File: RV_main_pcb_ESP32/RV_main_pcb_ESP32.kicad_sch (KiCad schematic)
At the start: 3 parts, among them J1 Conn_01x15_Female, J2 Conn_01x15_Female

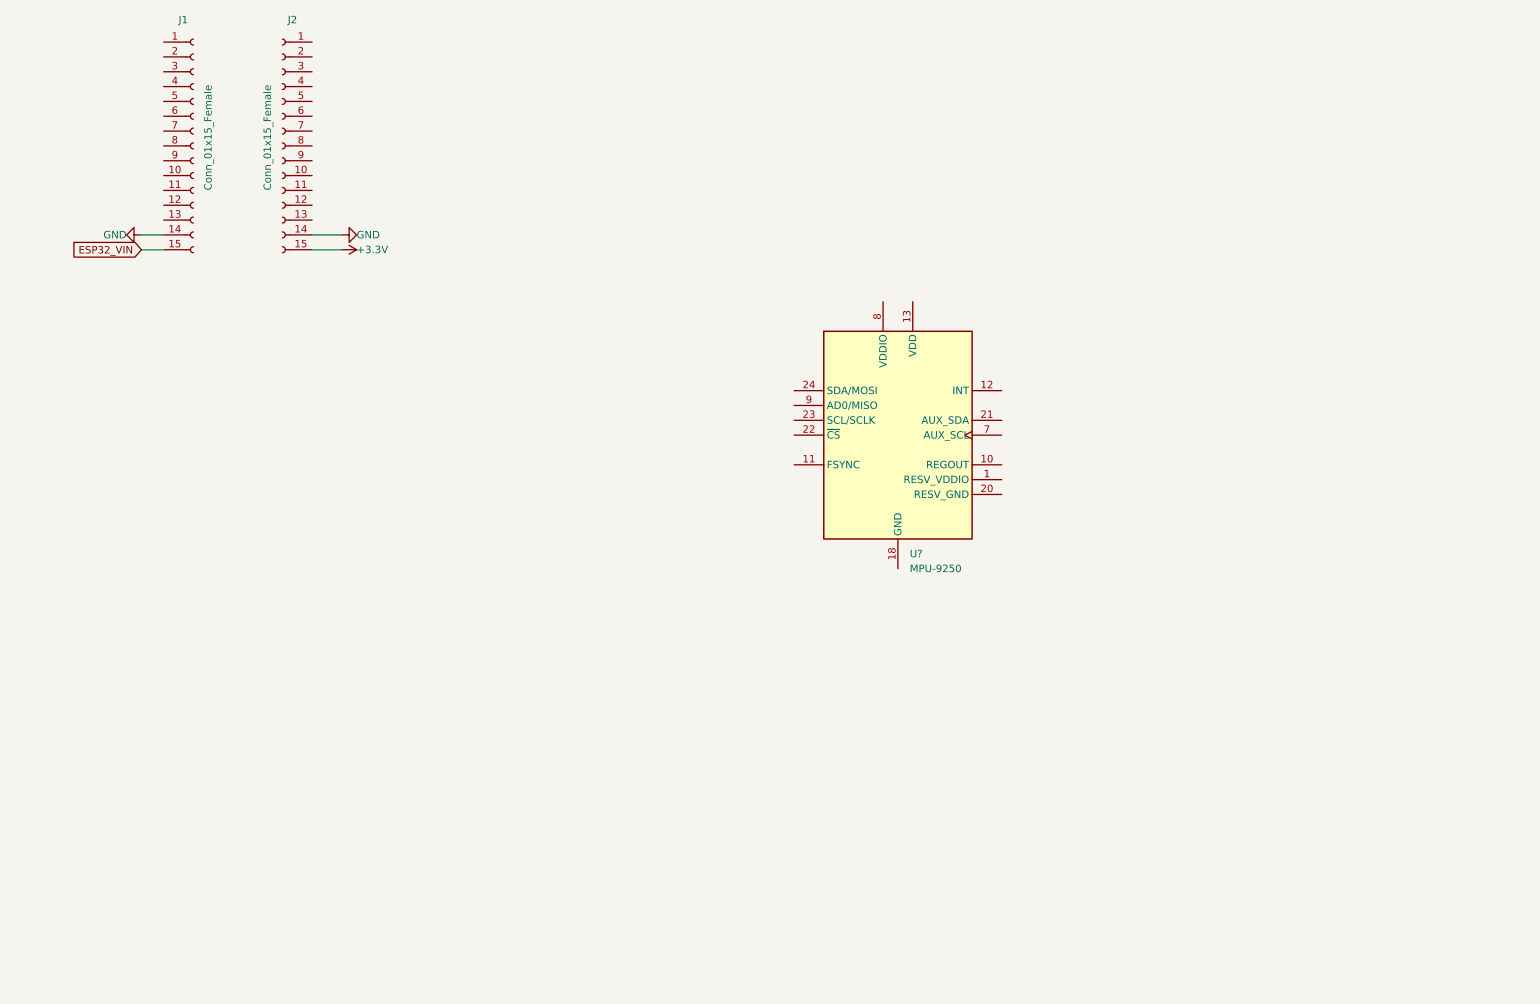
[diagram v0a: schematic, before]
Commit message: schematics
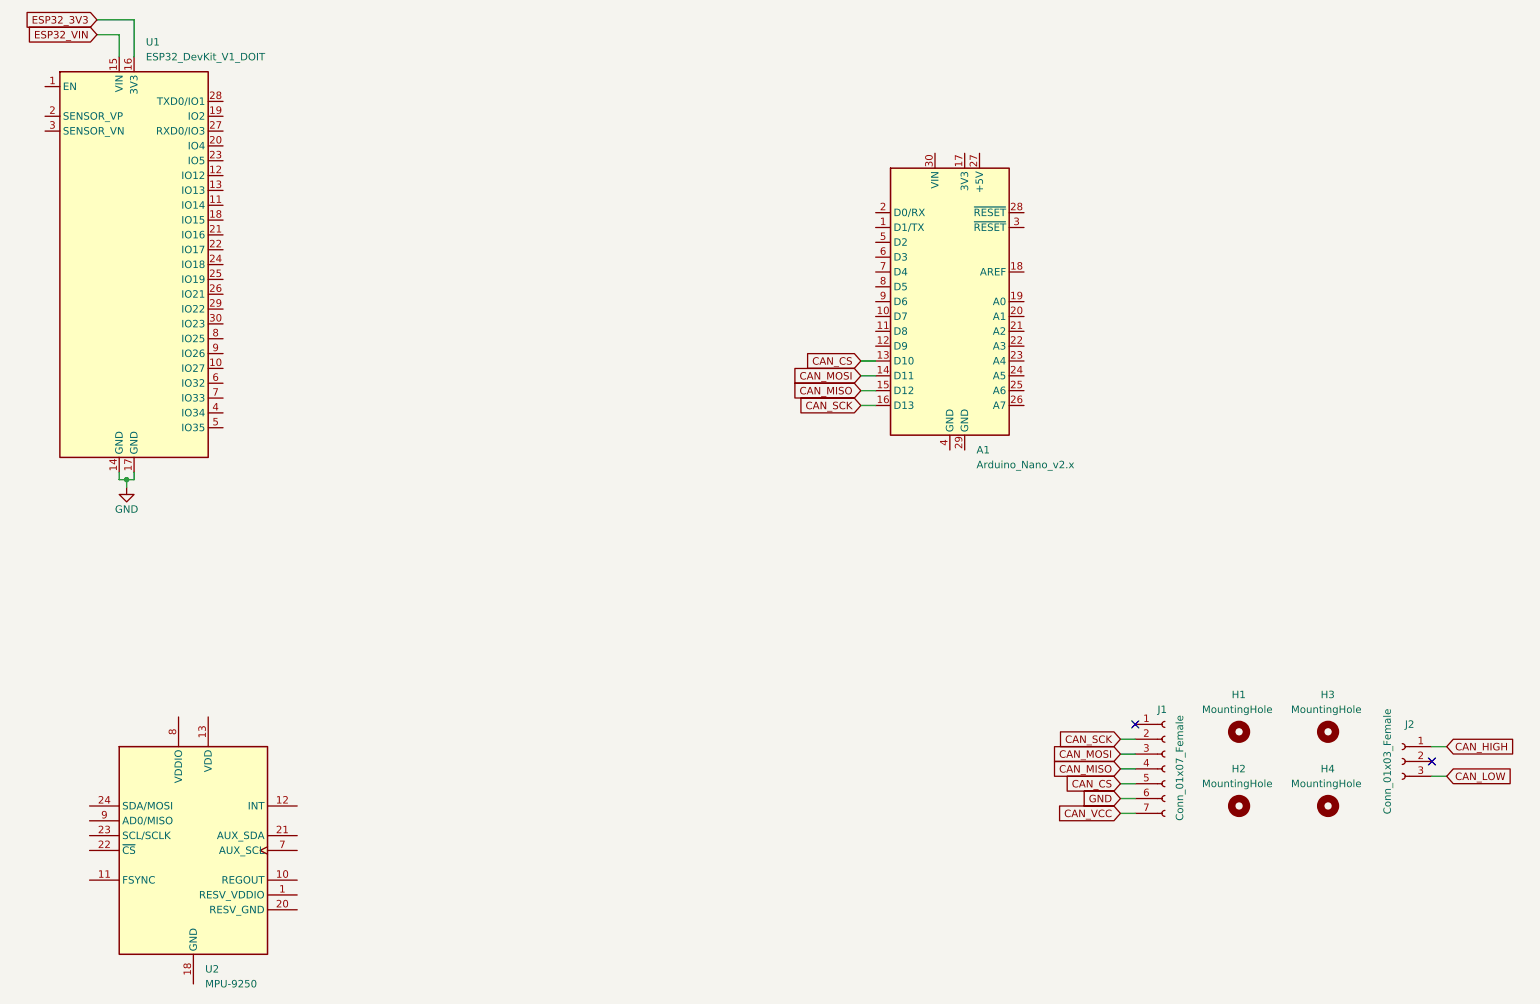
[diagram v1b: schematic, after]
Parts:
- removed J1, J2: Conn_01x15_Female, Connector_PinHeader_2.54mm:PinHeader_1x15_P2.54mm_Vertical, symbol Connector:Conn_01x15_Female
- added A1: Arduino_Nano_v2.x, Module:Arduino_Nano, symbol MCU_Module:Arduino_Nano_v2.x
- added H1, H2, H3, H4: MountingHole, MountingHole:MountingHole_3.2mm_M3_ISO7380, symbol Mechanical:MountingHole
- added J1: Conn_01x07_Female, Connector_PinHeader_2.54mm:PinHeader_1x06_P2.54mm_Vertical, symbol Connector:Conn_01x07_Female
- added J2: Conn_01x03_Female, Connector_PinHeader_2.54mm:PinHeader_1x03_P2.54mm_Vertical, symbol Connector:Conn_01x03_Female
- added U1: ESP32_DevKit_V1_DOIT, esp32_devkit_v1_doit:esp32_devkit_v1_doit, symbol esp32_devkit_v1_doit:ESP32_DevKit_V1_DOIT
- gave numbers to parts that had none: 1
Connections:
- net ESP32_VIN: now also U1.15 (VIN)
- net GND: now also J1.6 (Pin_6), U1.14 (GND), U1.17 (GND)
- new net CAN_CS: A1.13 (D10), J1.5 (Pin_5)
- new net CAN_HIGH: J2.1 (Pin_1)
- new net CAN_LOW: J2.3 (Pin_3)
- new net CAN_MISO: A1.15 (D12), J1.4 (Pin_4)
- new net CAN_MOSI: A1.14 (D11), J1.3 (Pin_3)
- new net CAN_SCK: A1.16 (D13), J1.2 (Pin_2)
- new net CAN_VCC: J1.7 (Pin_7)
- new net ESP32_3V3: U1.16 (3V3)
- no-connect marks 0 -> 2
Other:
- moved on the sheet: U2
